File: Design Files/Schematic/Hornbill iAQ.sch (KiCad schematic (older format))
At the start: 11 parts, among them U1 ESP32_Breakout1, U2 iAQCOREC, U3 OLED_I2C

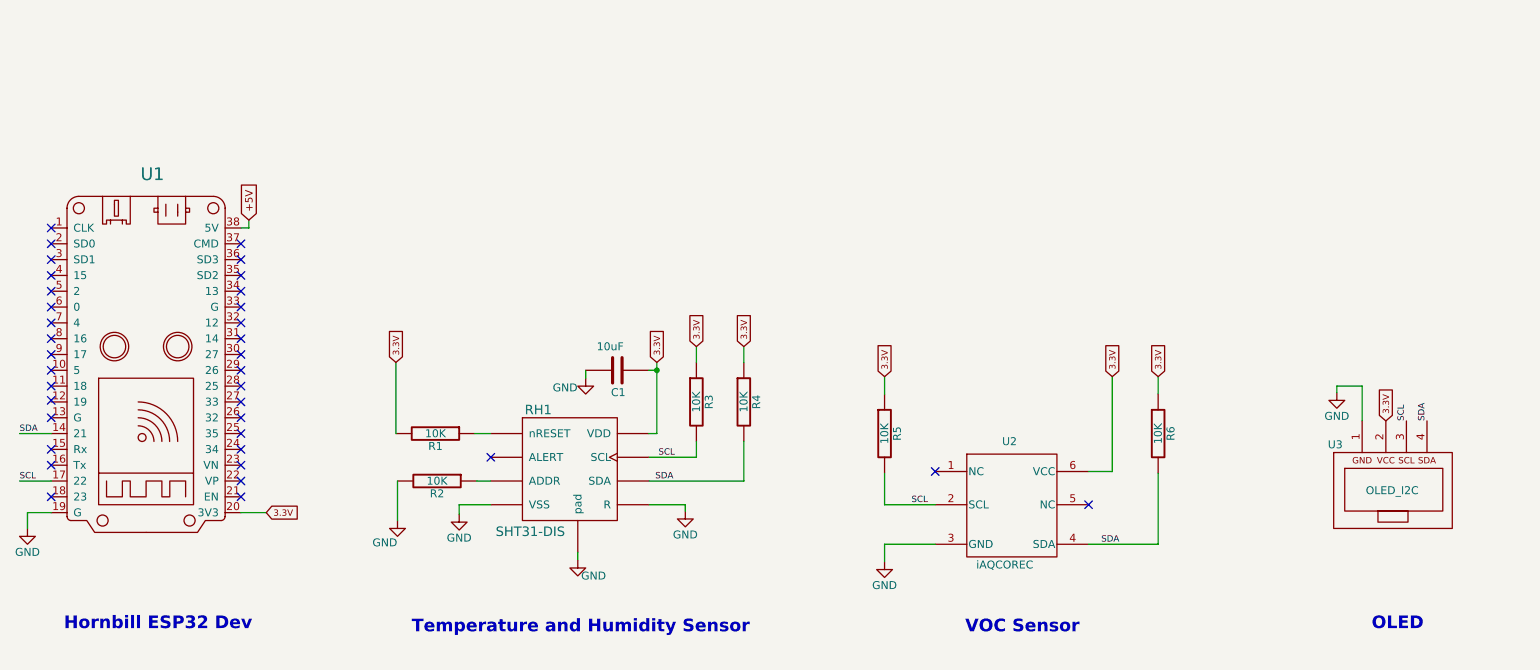
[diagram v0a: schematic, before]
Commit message: Schematic modified and Case design file added
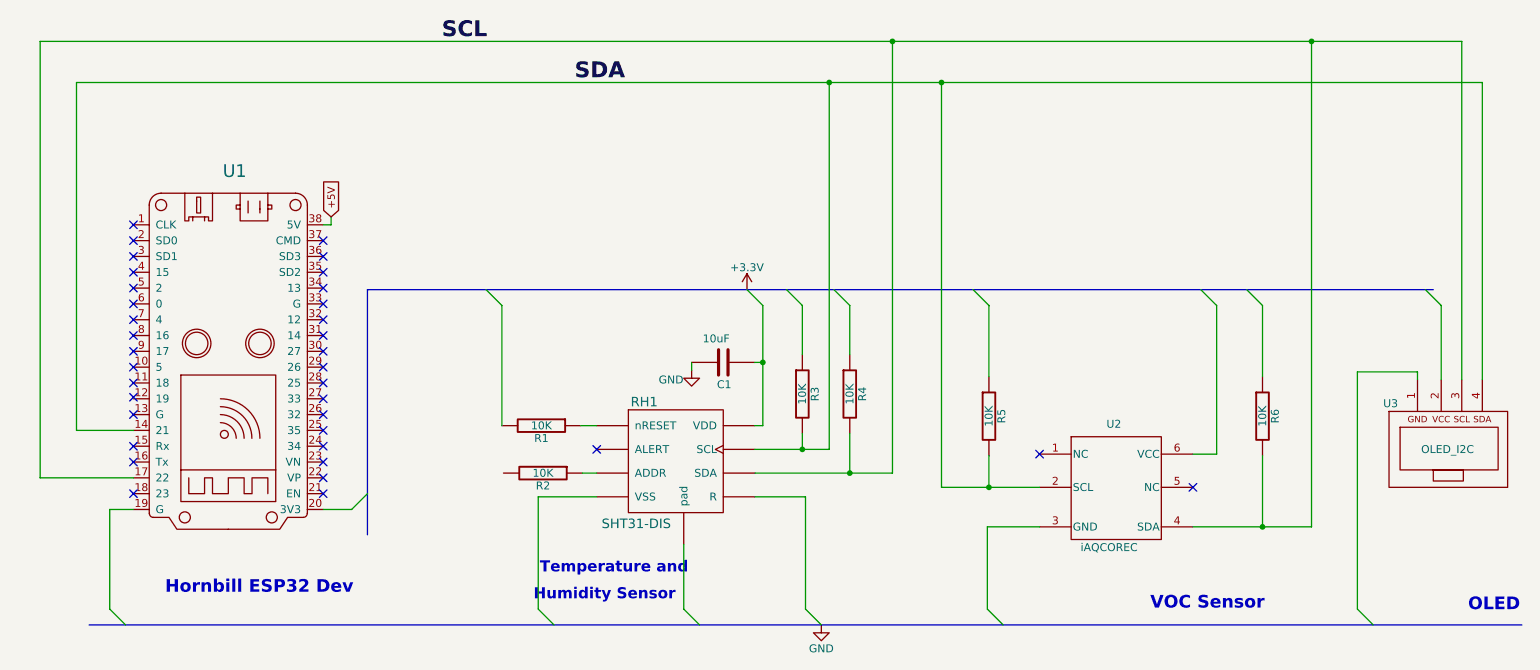
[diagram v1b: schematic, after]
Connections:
- net GND: no longer R2.2, RH1.7 (R), RH1.8 (VSS), RH1.9 (pad), U1.19 (G), U2.3 (GND), U3.1
- net SCL: now also R4.2, R6.2, RH1.1 (SDA), U2.4 (SDA); no longer R3.2, R5.2, RH1.4 (SCL), U2.2 (SCL)
- net SDA: now also R3.2, R5.2, RH1.4 (SCL), U2.2 (SCL); no longer R4.2, R6.2, RH1.1 (SDA), U2.4 (SDA)
- removed net 3.3V: C1.1, R1.2, R3.1, R4.1, R5.1, R6.1, RH1.5 (VDD), U1.20 (3V3), U2.6 (VCC), U3.2
- new net: C1.1, RH1.5 (VDD)
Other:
- note added: "Humidity Sensor"
- note added: "Temperature and"
- note removed: "Temperature and Humidity Sensor"
- moved on the sheet: C1, R1, R2, R3, R4, R5, R6, RH1, U1, U2, U3
